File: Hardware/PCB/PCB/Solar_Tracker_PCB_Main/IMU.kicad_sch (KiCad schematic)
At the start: 1 part, among them IC3 BNO085

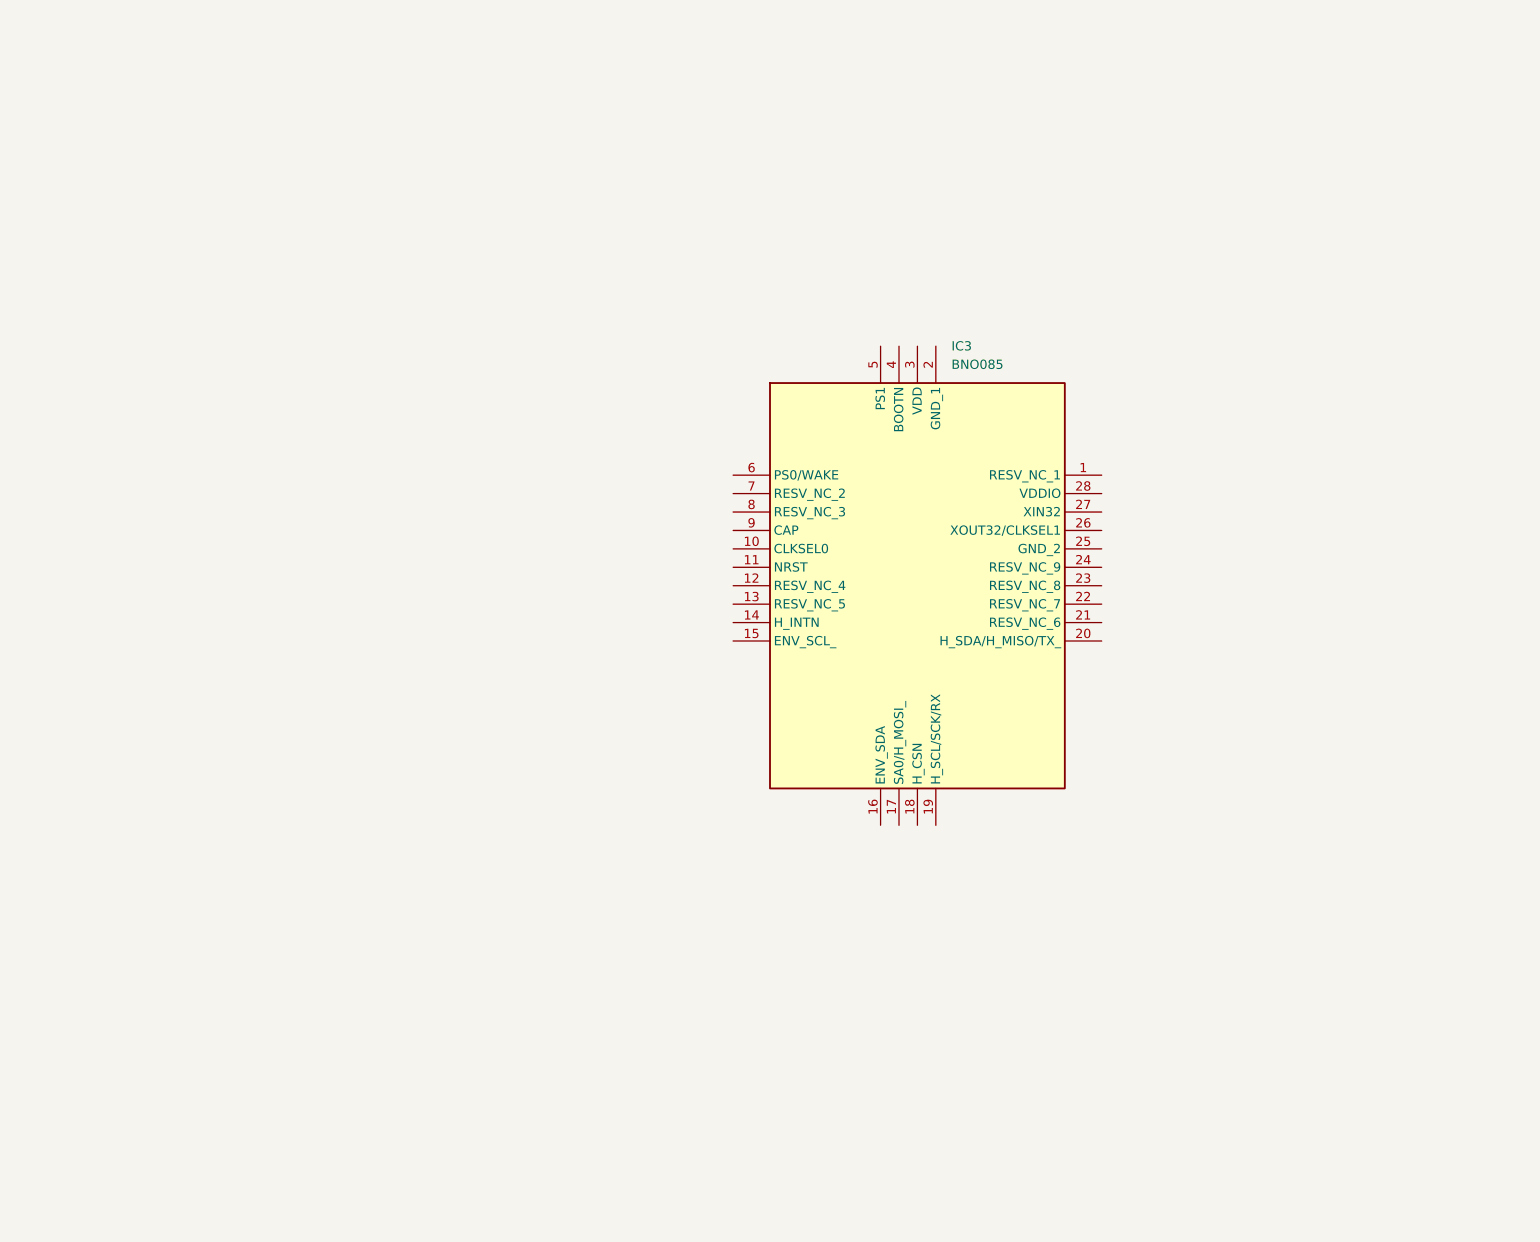
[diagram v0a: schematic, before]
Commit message: actualizacion de pcb (IMU)
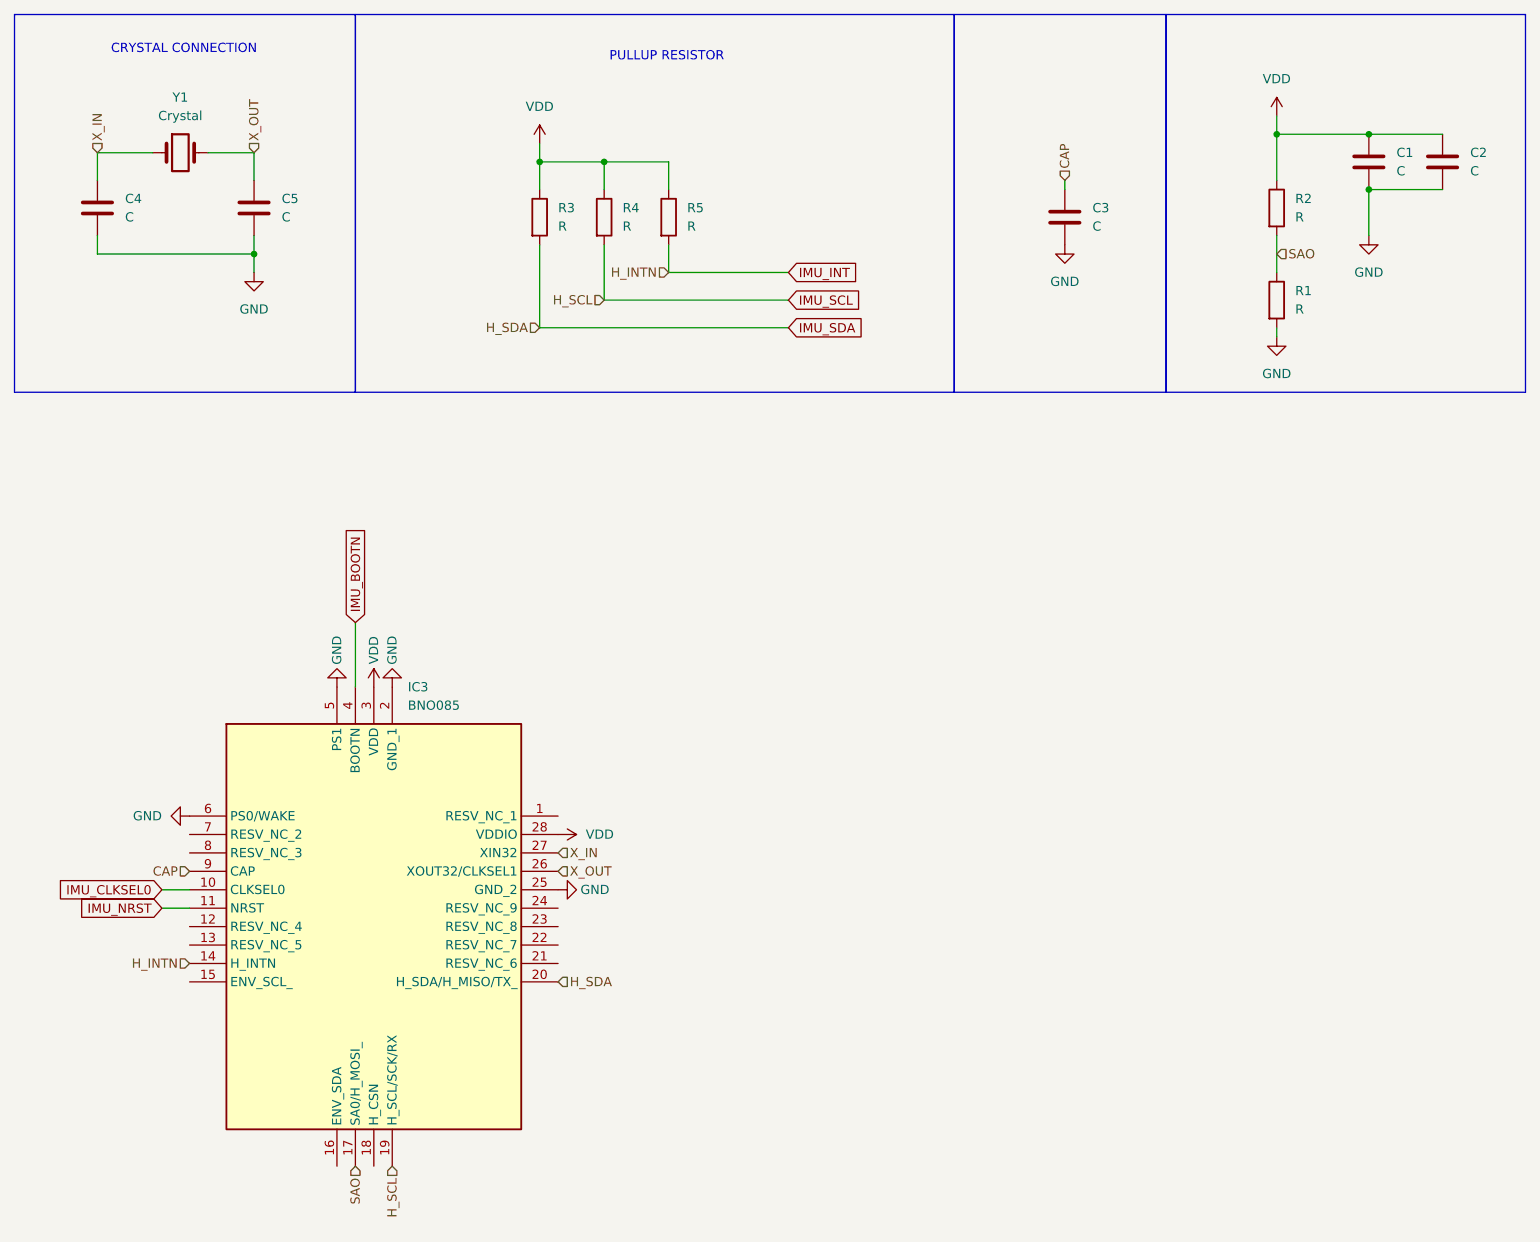
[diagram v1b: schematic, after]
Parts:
- added C1, C2, C3, C4, C5: C, symbol Device:C
- added R1, R2, R3, R4, R5: R, symbol Device:R
- added Y1: Crystal, symbol Device:Crystal
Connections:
- net IMU_CLKSEL0: now reaches IC3.10 (CLKSEL0)
- net IMU_NRST: now reaches IC3.11 (NRST)
- net IMU_INT: now reaches IC3.14 (H_INTN)
- net IMU_INT: now also R5.2
- net SAO: now reaches IC3.17 (SA0/H_MOSI_)
- net SAO: now also R1.1, R2.2
- net IMU_SCL: now reaches IC3.19 (H_SCL/SCK/RX)
- net IMU_SCL: now also R4.2
- net GND: now reaches IC3.2 (GND_1)
- net GND: now also IC3.25 (GND_2), IC3.5 (PS1), IC3.6 (PS0/WAKE), C1.2, C2.2, C3.2, C4.2, C5.2, R1.2
- net IMU_SDA: now reaches IC3.20 (H_SDA/H_MISO/TX_)
- net IMU_SDA: now also R3.2
- net X_OUT: now reaches IC3.26 (XOUT32/CLKSEL1)
- net X_OUT: now also C5.1, Y1.2
- net X_IN: now reaches IC3.27 (XIN32)
- net X_IN: now also C4.1, Y1.1
- net VDD: now reaches IC3.28 (VDDIO)
- net VDD: now also IC3.3 (VDD), C1.1, C2.1, R2.1, R3.1, R4.1, R5.1
- net IMU_BOOTN: now reaches IC3.4 (BOOTN)
- net CAP: now reaches IC3.9 (CAP)
- net CAP: now also C3.1
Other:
- note added: "CRYSTAL CONNECTION"
- note added: "PULLUP RESISTOR"
- moved on the sheet: IC3
